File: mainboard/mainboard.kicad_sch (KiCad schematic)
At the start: 15 parts

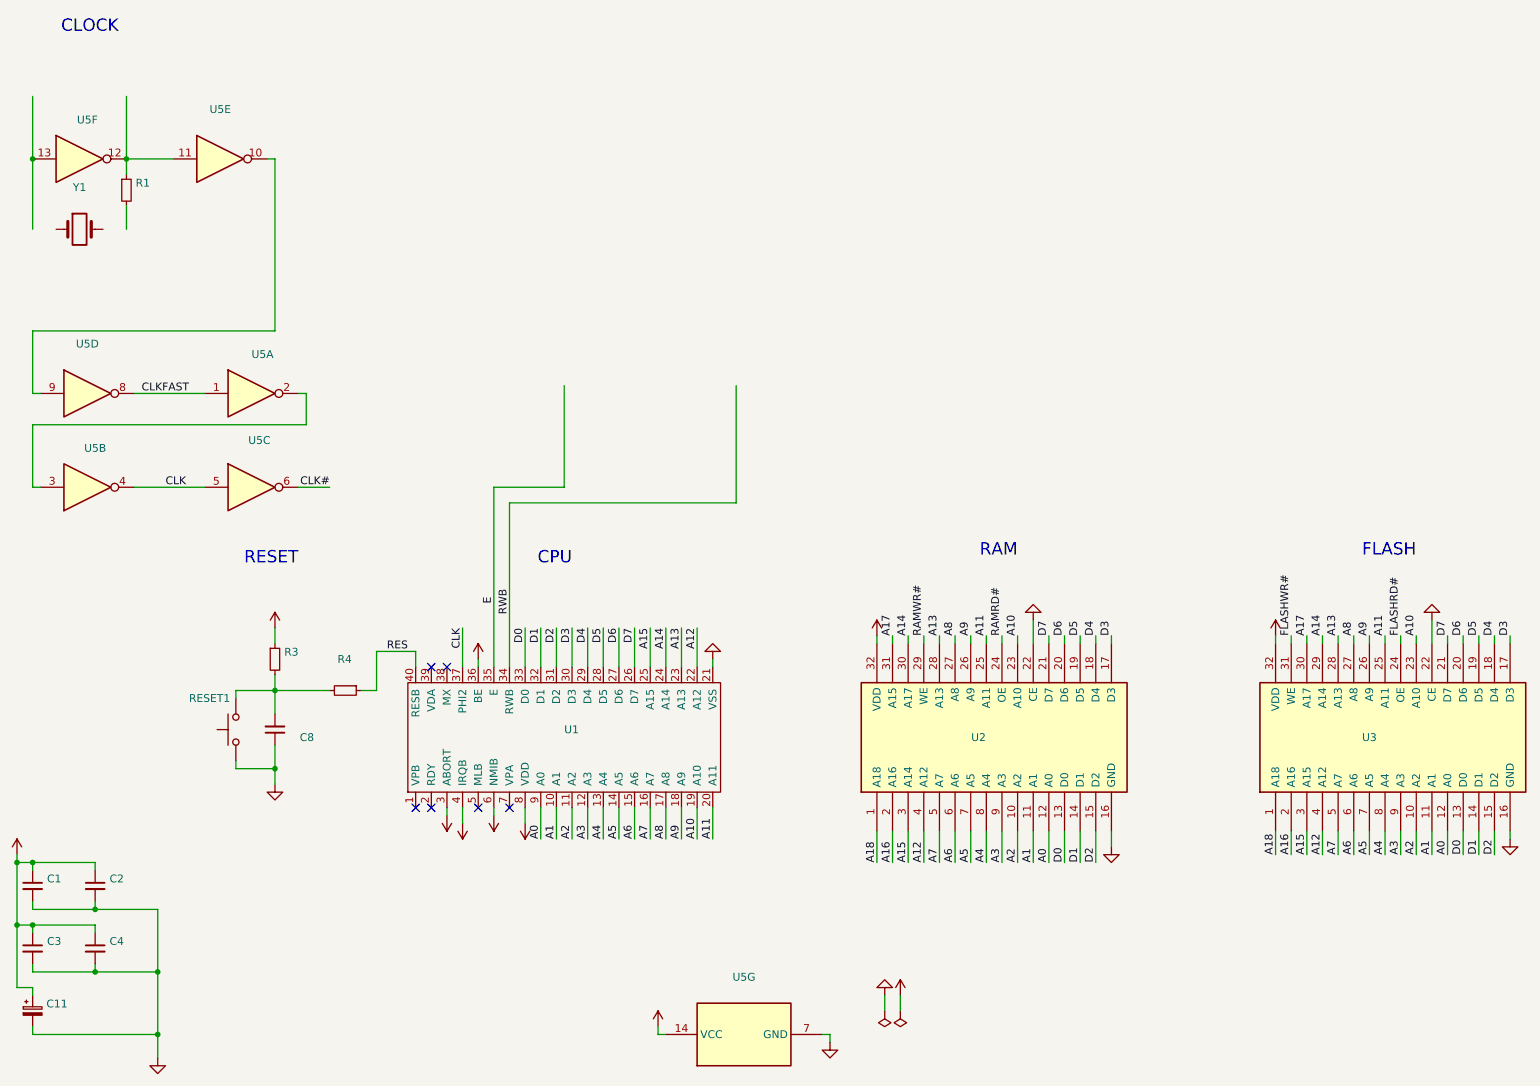
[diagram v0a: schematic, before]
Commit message: Schematic
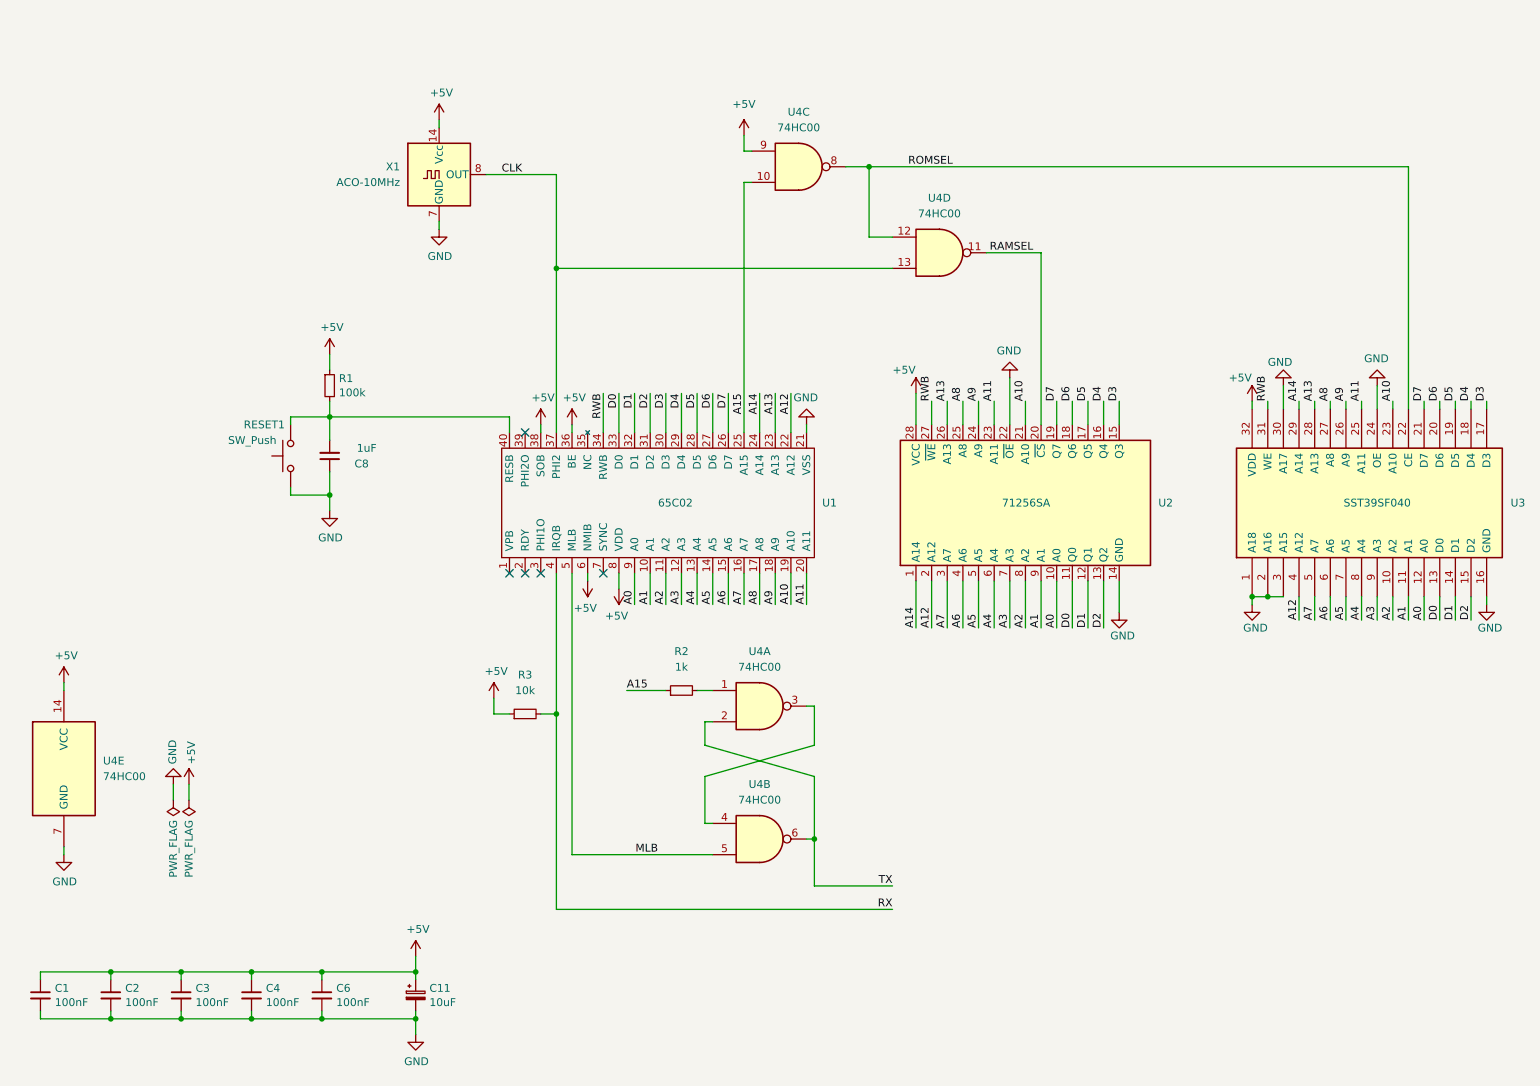
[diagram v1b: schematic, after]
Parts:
- removed R1, R4: (no value), symbol Device:R_Small
- removed U1: (no value), symbol mainboard-rescue:65C816-Library
- removed U2: (no value), symbol parts:AS6C4008
- removed U5: (no value), symbol 74xx:74HC04
- removed Y1: (no value), symbol Device:Crystal
- added C6: 100nF, Capacitor_THT:C_Disc_D3.0mm_W2.0mm_P2.50mm, symbol Device:C_Small
- added R2: 1k, symbol Device:R_Small
- added R3: 10k, symbol Device:R_Small
- added U1: 65C02, Package_DIP:DIP-40_W15.24mm_Socket, symbol library:65C02
- added U2: 71256SA, Package_DIP:DIP-28_W15.24mm, symbol library:71256SA
- added U4: 74HC00, symbol 74xx:74HC00
- added X1: ACO-10MHz, Oscillator:Oscillator_DIP-14, symbol Oscillator:ACO-xxxMHz
- C1, C2, C3, C4: value (none) -> 100nF; footprint (none) -> Capacitor_THT:C_Disc_D3.0mm_W2.0mm_P2.50mm
- C11: value (none) -> 10uF; footprint (none) -> Capacitor_THT:CP_Radial_D5.0mm_P2.50mm
- C8: value (none) -> 1uF; footprint (none) -> Capacitor_THT:C_Disc_D3.0mm_W2.0mm_P2.50mm
- R1: renamed from R3; value (none) -> 100k; footprint (none) -> Resistor_THT:R_Axial_DIN0207_L6.3mm_D2.5mm_P7.62mm_Horizontal
- RESET1: value (none) -> SW_Push; footprint (none) -> Button_Switch_THT:SW_PUSH_6mm_H4.3mm
- U3: value (none) -> SST39SF040; footprint (none) -> Package_DIP:DIP-32_W15.24mm_Socket
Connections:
- net A16 is gone; now on net GND: U3.2 (A16)
- net A17 is gone; now on net GND: U3.30 (A17)
- net A18 is gone; now on net GND: U3.1 (A18)
- net FLASHRD# is gone; now on net GND: U3.24 (OE)
- net FLASHWR# is gone; now on net RWB: U3.31 (WE)
- net +5V: now also C6.1, R3.1, U1.36 (BE), U1.38 (SOB), U1.6 (NMIB), U1.8 (VDD), U2.28 (VCC), U4.14 (VCC), U4.9, X1.14 (Vcc)
- net A0: now also U1.9 (A0), U2.10 (A0)
- net A1: now also U1.10 (A1), U2.9 (A1)
- net A10: now also U1.19 (A10), U2.21 (A10)
- net A11: now also U1.20 (A11), U2.23 (A11)
- net A12: now also U1.22 (A12), U2.2 (A12)
- net A13: now also U1.23 (A13), U2.26 (A13)
- net A14: now also U1.24 (A14), U2.1 (A14)
- net A15: now also R2.1, U1.25 (A15), U4.10; no longer U3.3 (A15)
- net A2: now also U1.11 (A2), U2.8 (A2)
- net A3: now also U1.12 (A3), U2.7 (A3)
- net A4: now also U1.13 (A4), U2.6 (A4)
- net A5: now also U1.14 (A5), U2.5 (A5)
- net A6: now also U1.15 (A6), U2.4 (A6)
- net A7: now also U1.16 (A7), U2.3 (A7)
- net A8: now also U1.17 (A8), U2.25 (A8)
- net A9: now also U1.18 (A9), U2.24 (A9)
- net CLK: now also U1.37 (PHI2), U4.13, X1.8 (OUT)
- net D0: now also U1.33 (D0), U2.11 (Q0)
- net D1: now also U1.32 (D1), U2.12 (Q1)
- net D2: now also U1.31 (D2), U2.13 (Q2)
- net D3: now also U1.30 (D3), U2.15 (Q3)
- net D4: now also U1.29 (D4), U2.16 (Q4)
- net D5: now also U1.28 (D5), U2.17 (Q5)
- net D6: now also U1.27 (D6), U2.18 (Q6)
- net D7: now also U1.26 (D7), U2.19 (Q7)
- net GND: now also U3.3 (A15), C6.2, U1.21 (VSS), U2.14 (GND), U2.22 (~{OE}), U4.7 (GND), X1.7 (GND); no longer U3.22 (CE)
- net RWB: now also U1.34 (RWB), U2.27 (~{WE})
- net at C8.2, R1.2, RESET1.2: now also U1.40 (RESB)
- new net: U4.3, U4.4
- new net: R2.2, U4.1
- new net MLB: U1.5 (MLB), U4.5
- new net RAMSEL: U2.20 (~{CS}), U4.11
- new net ROMSEL: U3.22 (CE), U4.12, U4.8
- new net RX: R3.2, U1.4 (IRQB)
- new net TX: U4.2, U4.6
- no-connect marks 6 -> 5
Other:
- note removed: "CLOCK"
- note removed: "CPU"
- note removed: "FLASH"
- note removed: "RAM"
- note removed: "RESET"
- title: OS816 computer -> SingleBreadboardComputer
- moved on the sheet: C1, C11, C2, C3, C4, C8, R1, RESET1, U3
